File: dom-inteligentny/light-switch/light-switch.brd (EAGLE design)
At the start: 92.7 x 87.6 mm, 25 parts, among them X1 GLX-S-88M, X10 TERMINAL-BLOCK-3.5MM-4-PIN-LO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, X11 TERMINAL-BLOCK-3.5MM-4-PIN-LO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, X12 TERMINAL-BLOCK-3.5MM-2-PIN-LO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, X13 TERMINAL-BLOCK-3.5MM-2-PIN-LO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, X2 TERMINAL-BLOCK-3.5MM-3-PIN-LO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, X3 TERMINAL-BLOCK-3.5MM-3-PIN-LO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, X4 TERMINAL-BLOCK-3.5MM-4-PIN-LO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, X5 TERMINAL-BLOCK-3.5MM-2-PIN-LO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, X6 TERMINAL-BLOCK-3.5MM-4-PIN-LO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, X7 TERMINAL-BLOCK-3.5MM-2-PIN-LO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, X8 TERMINAL-BLOCK-3.5MM-2-PIN-LO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, X9 TERMINAL-BLOCK-3.5MM-2-PIN-LO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

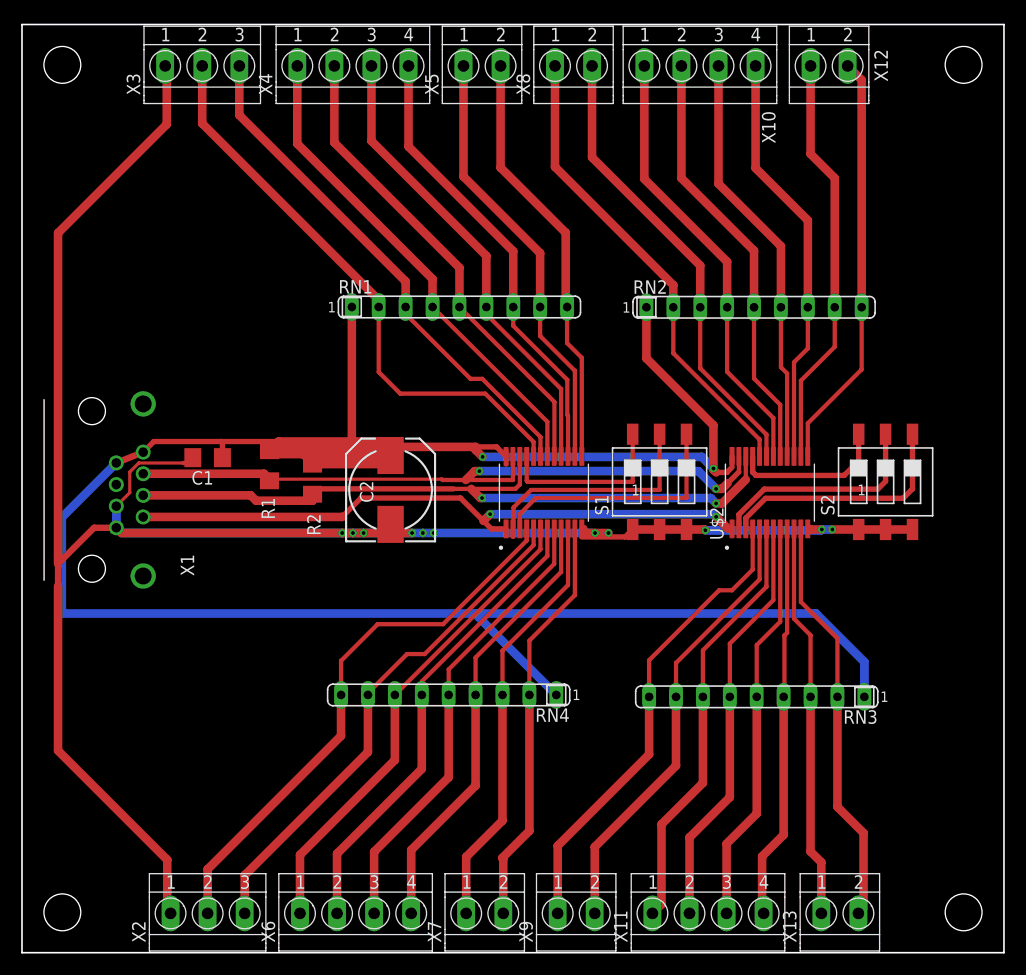
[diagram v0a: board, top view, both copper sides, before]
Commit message: new files
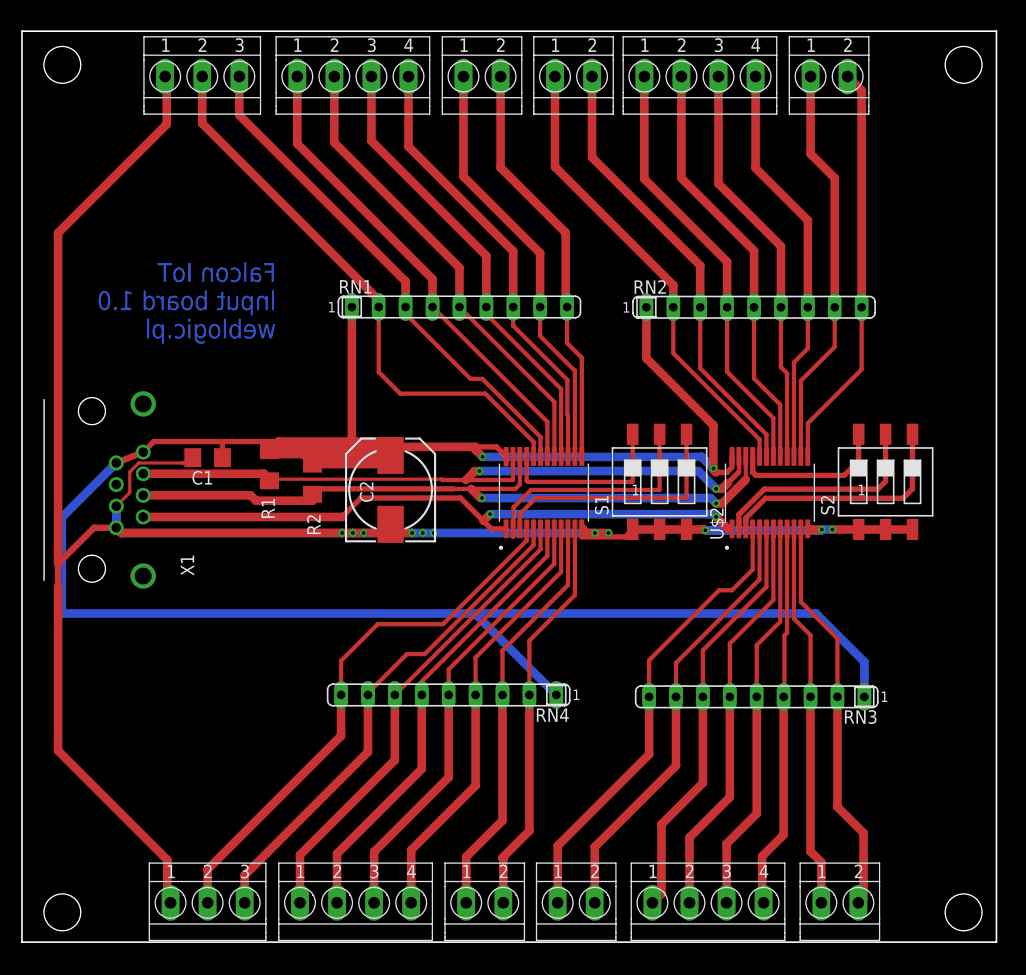
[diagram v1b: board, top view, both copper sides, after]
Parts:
- moved X10 1.00 mm to (64.0, 82.8)
- moved X12 1.00 mm to (76.2, 82.8)
- moved X3 1.00 mm to (17.0, 82.8)
- moved X4 1.00 mm to (31.2, 82.8)
- moved X5 1.00 mm to (43.4, 82.8)
- moved X8 1.00 mm to (52.1, 82.8)
- moved X11 1.00 mm to (64.8, 4.81)
- moved X13 1.00 mm to (77.2, 4.81)
- moved X2 1.00 mm to (17.5, 4.81)
- moved X6 1.00 mm to (31.5, 4.81)
- moved X7 1.00 mm to (43.7, 4.81)
- moved X9 1.00 mm to (52.3, 4.81)
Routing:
- net GND: track 225.6 -> 223.6 mm
- net N$9: track 40.0 -> 39.0 mm
- net N$8: track 41.4 -> 40.4 mm
- net N$7: track 43.1 -> 42.1 mm
- net N$6: track 44.3 -> 43.3 mm
- net N$5: track 45.5 -> 44.5 mm
- net N$45: track 39.0 -> 38.0 mm
- net N$44: track 37.4 -> 36.4 mm
- net N$43: track 37.3 -> 36.3 mm
- net N$42: track 38.4 -> 37.4 mm
- net N$41: track 39.6 -> 38.6 mm
- net N$40: track 40.8 -> 39.8 mm
- net N$4: track 46.6 -> 45.6 mm
- net N$39: track 42.8 -> 41.8 mm
- net N$36: track 39.1 -> 38.1 mm
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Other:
- board size 92.7 x 87.6 mm -> 92 x 86 mm
- board text added: "Falcon IoT lnput board 1.0 weblogic.pl"
